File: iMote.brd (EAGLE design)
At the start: 43 x 50 mm, 48 parts, among them CN1 USB-MINIB-UX60SC-MB, CN2 ICSP, CN3 CC-HEADER, IC1 ATmega328P-AU, IC2 FT232RLSSOP, IC3 BLE112-A-VISUAL, Q1 16MHz, T1 2SC1815

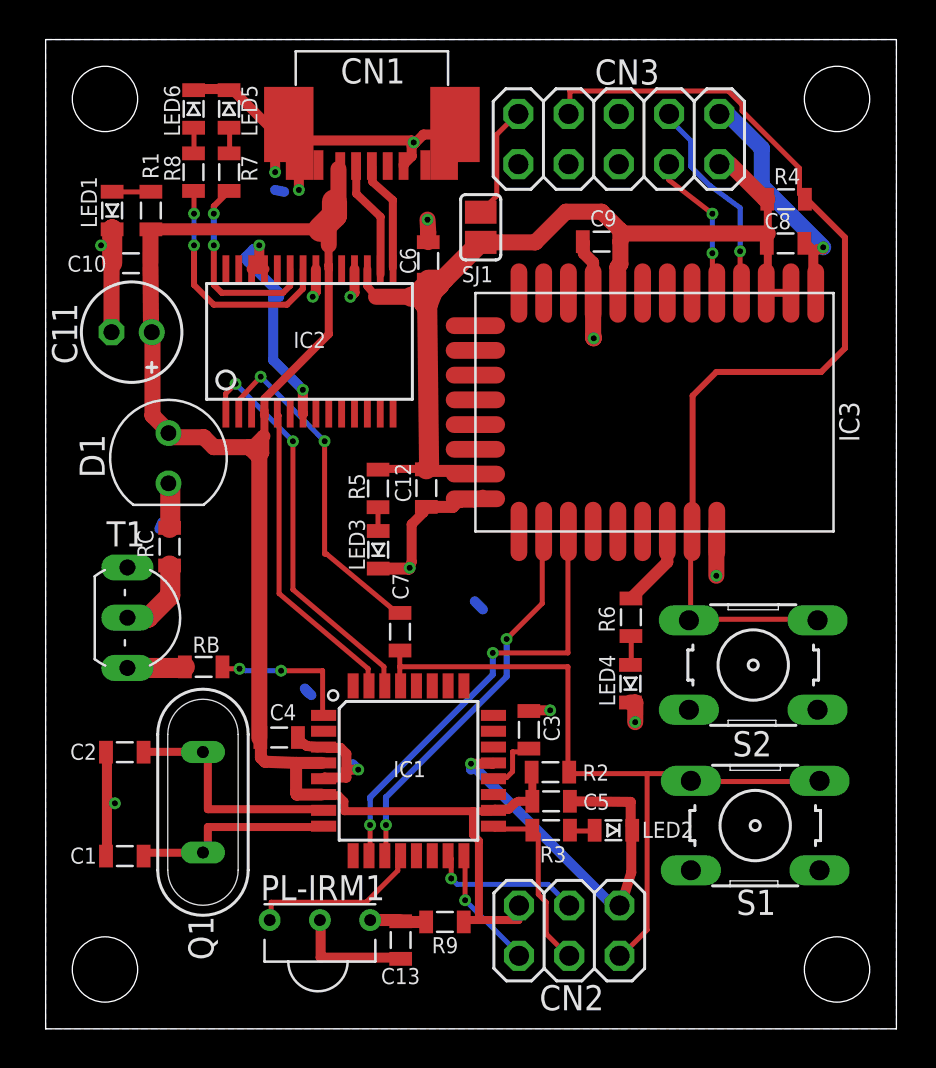
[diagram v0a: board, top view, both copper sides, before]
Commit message: もろもろ余裕を出そうとしている
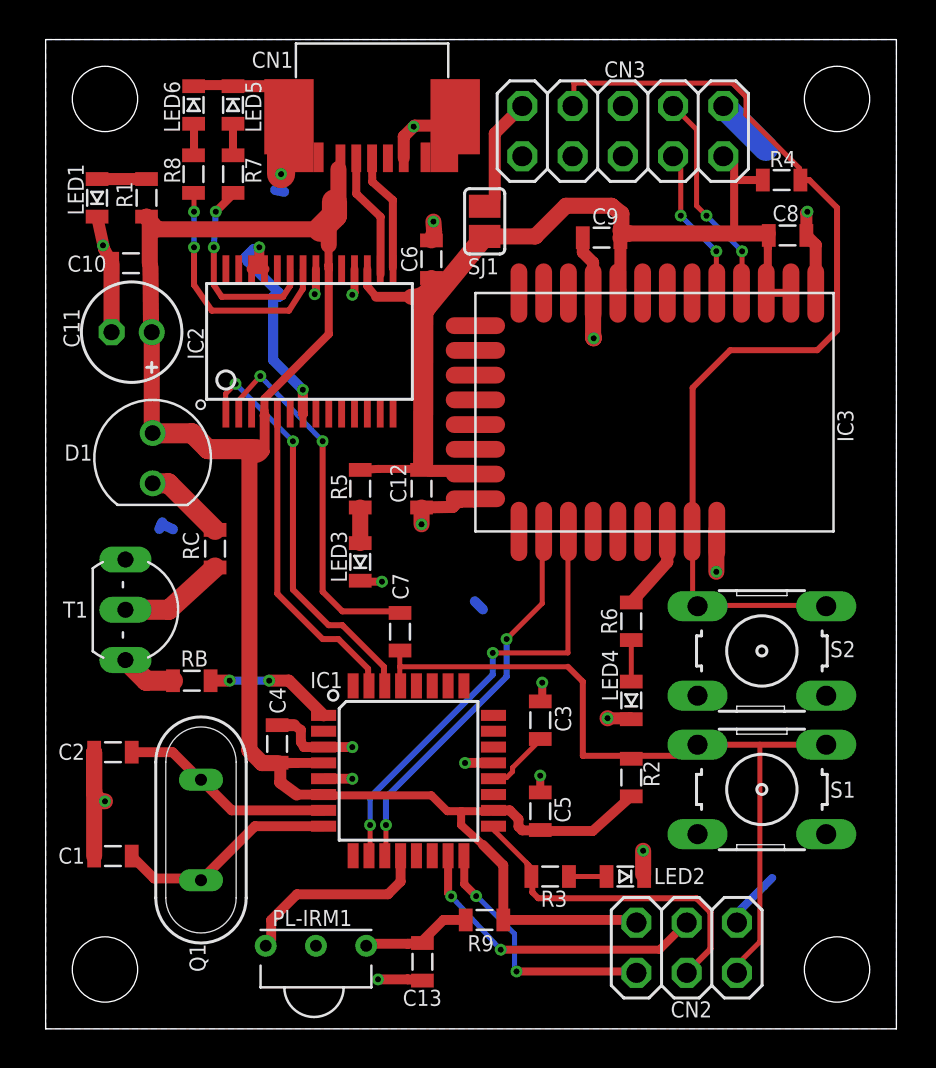
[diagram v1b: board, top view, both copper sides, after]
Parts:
- moved CN2 6.00 mm to (32.4, 4.10)
- moved R2 4.10 mm to (29.6, 12.7), turned to 270 degrees
- moved LED2 2.41 mm to (29.3, 7.70)
- moved R3 2.34 mm to (25.5, 7.70)
- moved RC 2.30 mm to (8.56, 24.3)
- moved R9 2.00 mm to (22.2, 5.50)
- moved S1 1.86 mm to (36.2, 12.1)
- moved C13 1.56 mm to (19.0, 3.39)
- moved Q1 1.40 mm to (7.85, 10.1)
- moved PL-IRM1 1.32 mm to (13.7, 4.20)
- moved LED3 1.10 mm to (15.9, 23.6)
- moved R4 1.00 mm to (37.2, 42.9)
- moved LED1 1.00 mm to (2.60, 42.0)
- moved RB 0.92 mm to (7.39, 17.6)
- moved R5 0.90 mm to (15.9, 27.3)
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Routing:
- net GND: track 117.8 -> 86.4 mm, vias 18 -> 22
- net +5V: track 85.9 -> 98.8 mm
- net D13/SCK: track 9.31 -> 18.5 mm
- net D11/MOSI: track 7.75 -> 15.8 mm, vias 1 -> 2
- net D12/MISO: track 6.31 -> 13.2 mm, vias 1 -> 2
- net +3V3: track 54.2 -> 60.1 mm
- net N$16: track 2.87 -> 5.71 mm
- net N$12: track 2.31 -> 4.13 mm
- net N$8: track 17.8 -> 19.5 mm
- net D8/IRIN: track 8.85 -> 10.1 mm
- net N$11: track 4.16 -> 5.36 mm
- net !RESET: track 38.9 -> 40.1 mm
- net N$2: track 12.1 -> 11.1 mm
- net N$1: track 10.5 -> 11.4 mm
- net D3/IROUT: track 7.41 -> 6.52 mm
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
